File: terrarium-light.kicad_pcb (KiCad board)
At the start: 2 copper layers, 100 x 100 mm, 59 parts, among them J1 Conn_01x04_Pin, J2 USB_C_Receptacle_USB2.0_16P, Q1 UMH3N, SW1 RotaryEncoder_Switch_MP, U1 CH340C, U2 TPS61169DCKR, U3 TPS61169DCKR, U4 LM1117S-3.3, U6 ESP32-S3-MINI-1

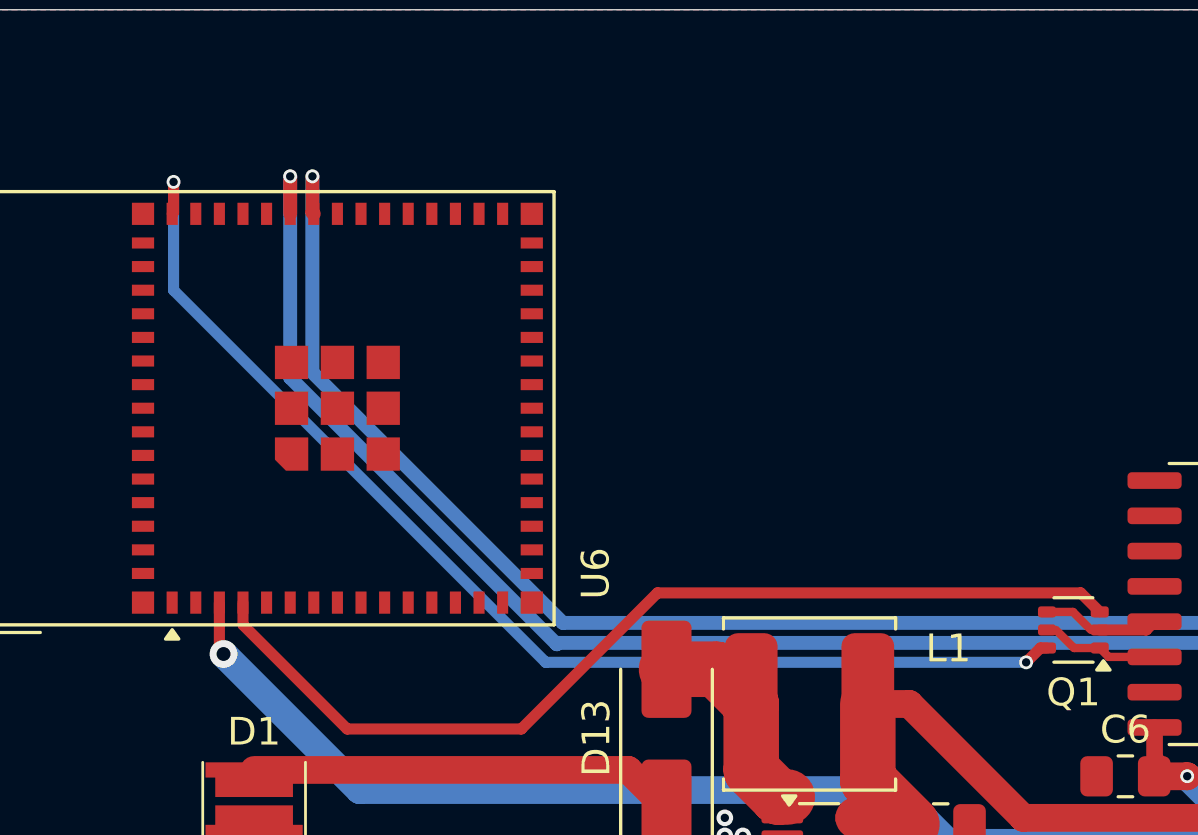
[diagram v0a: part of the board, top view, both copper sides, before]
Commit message: fixed
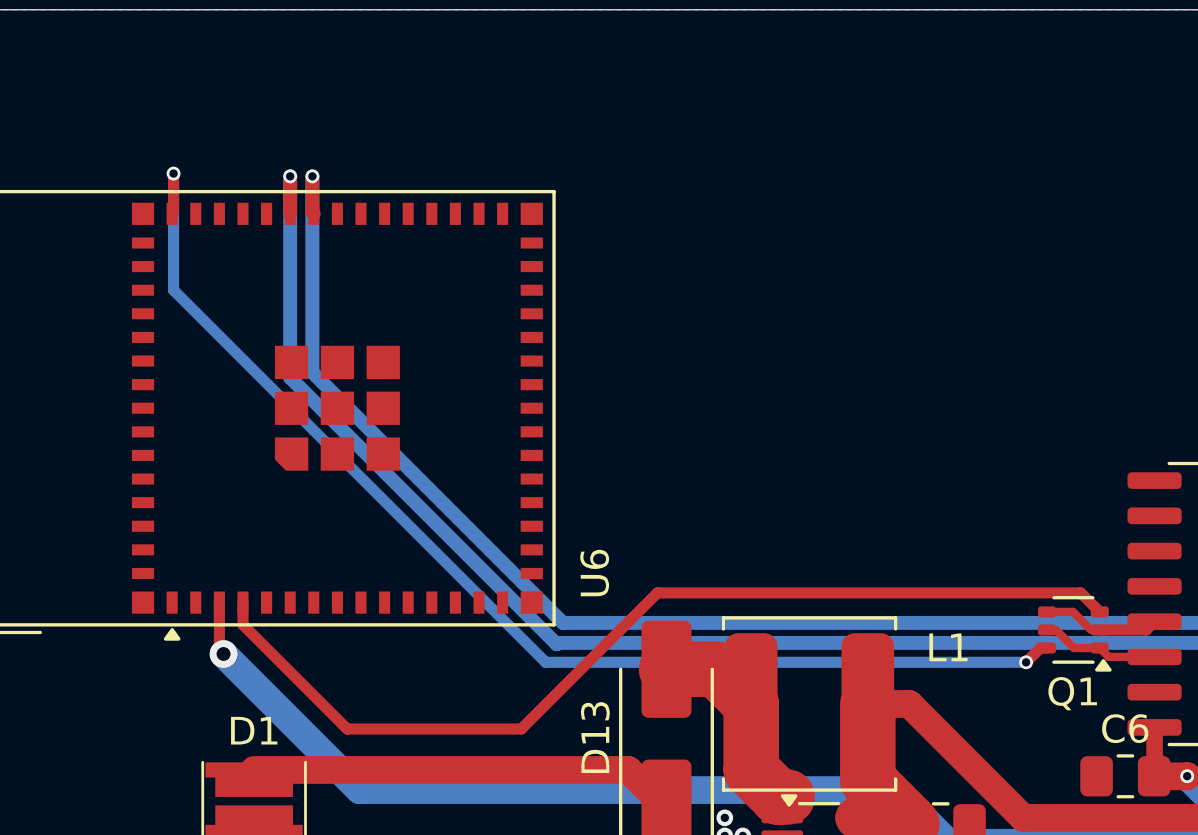
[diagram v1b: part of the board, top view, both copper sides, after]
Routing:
- net /ESP_EN: track 42.3 -> 42.9 mm
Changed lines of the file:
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@@
 				(font
 					(size 0.001 0.001)
+					(thickness 0.15)
 				)
 			)
@@
 				(font
 					(size 0.001 0.001)
+					(thickness 0.15)
 				)
 			)
@@
 	)
 	(segment
-		(start 57.1 57.3)
-		(end 57.05 57.35)
+		(start 57.1 55.9)
+		(end 57.1 57.3)
 		(width 0.4)
 		(layer "F.Cu")
@@
 	)
 	(segment
-		(start 57.1 56.2)
-		(end 57.1 57.3)
+		(start 57.1 57.3)
+		(end 57.05 57.35)
 		(width 0.4)
 		(layer "F.Cu")
@@
 	)
 	(via
-		(at 57.1 56.2)
+		(at 57.1 55.9)
 		(size 0.5)
 		(drill 0.3)
@@
 	)
 	(segment
-		(start 70.5 73.5)
+		(start 57.1 55.9)
 		(end 57.1 60.1)
 		(width 0.4)
@@
 	)
 	(segment
-		(start 87.8 73.5)
+		(start 57.1 60.1)
 		(end 70.5 73.5)
 		(width 0.4)
@@
 	)
 	(segment
-		(start 57.1 60.1)
-		(end 57.1 56.2)
+		(start 70.5 73.5)
+		(end 87.8 73.5)
 		(width 0.4)
 		(layer "B.Cu")
